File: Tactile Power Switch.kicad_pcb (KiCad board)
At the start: 2 copper layers, 24 x 26 mm, 12 parts, among them J1 OSTTC020162, J2 OSTTC020162, Q1 BC847B_215, Q2 BC847B_215, Q4 NDT2955

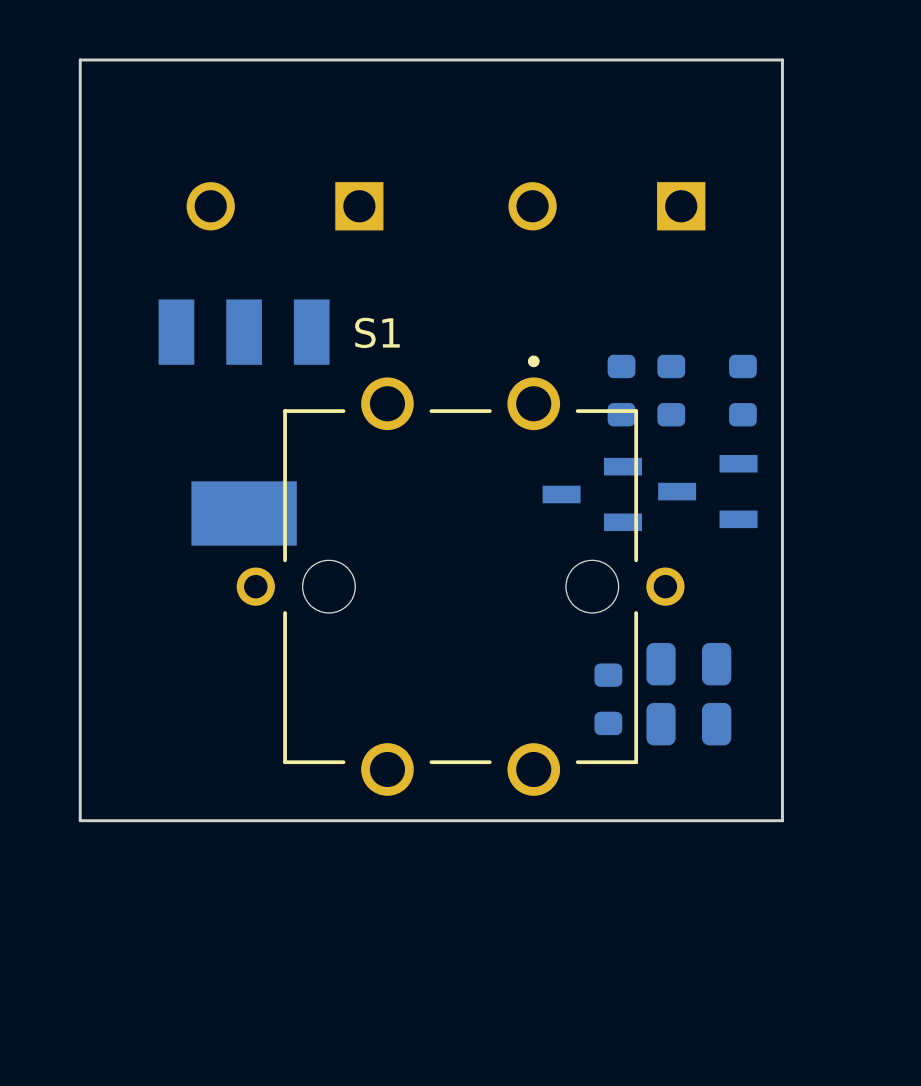
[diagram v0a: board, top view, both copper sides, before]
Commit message: Placement Finished
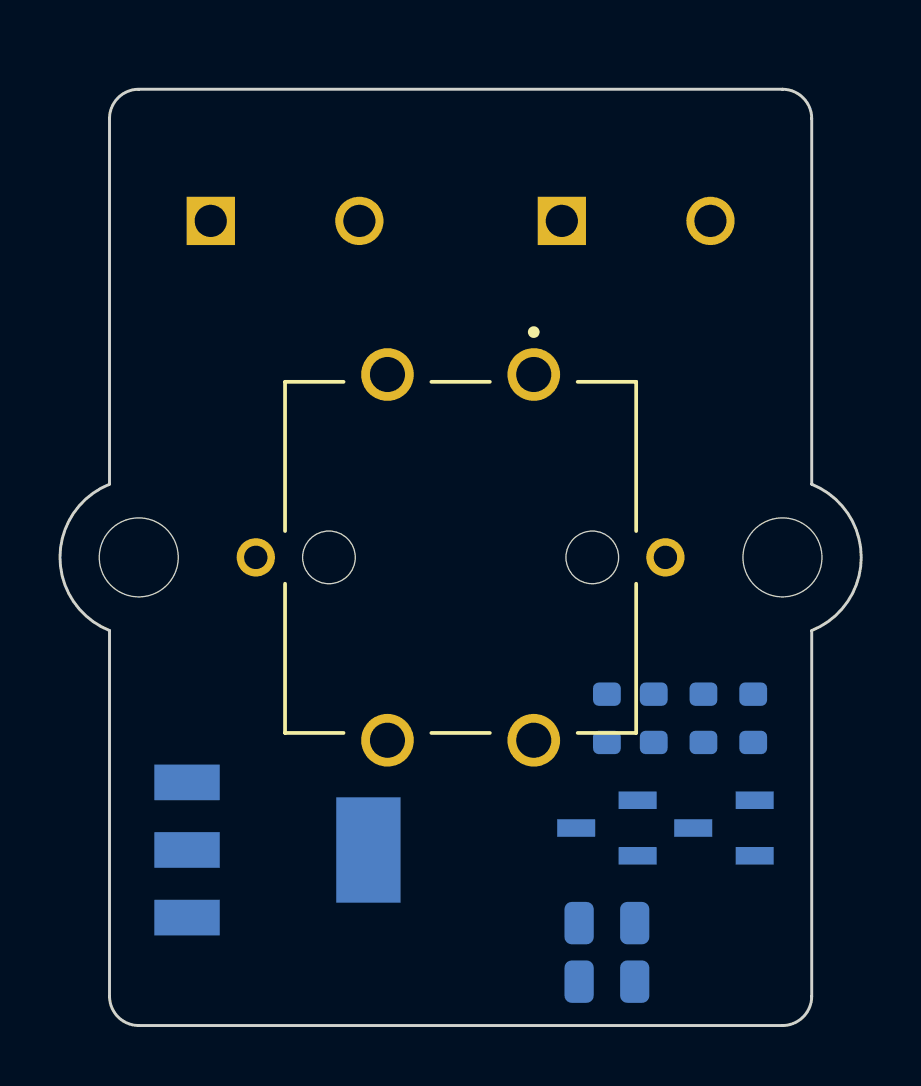
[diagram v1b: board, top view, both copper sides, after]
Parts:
- added H1: MountingHole, MountingHole:MountingHole_2.7mm_M2.5_ISO7380, F.Cu at (134.0, 62.0)
- added H2: MountingHole, MountingHole:MountingHole_2.7mm_M2.5_ISO7380, F.Cu at (112.0, 62.0)
- moved Q4 14.6 mm to (116.8, 72.0), turned to 90 degrees
- moved Q1 11.5 mm to (132.0, 71.2)
- moved Q2 11.4 mm to (128.0, 71.2)
- moved R1 11.3 mm to (131.3, 67.5)
- moved R3 11.3 mm to (129.6, 67.5)
- moved R2 11.2 mm to (133.0, 67.5)
- moved C1 9.28 mm to (128.0, 74.5)
- moved C2 9.23 mm to (128.0, 76.5)
- moved J2 1.12 mm to (129.0, 50.5), turned to 0 degrees
- moved S1 1.00 mm to (123.0, 62.0)
- moved R4 0.65 mm to (128.0, 67.5)
- moved J1 0.50 mm to (117.0, 50.5), turned to 0 degrees
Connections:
- net +5V renamed +12V
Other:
- board size 24 x 26 mm -> 27.4 x 32 mm
